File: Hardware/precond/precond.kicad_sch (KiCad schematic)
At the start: 21 parts, among them J1 Conn_Coaxial, J2 Conn_Coaxial, U1 OPA2340, U2 MAX660

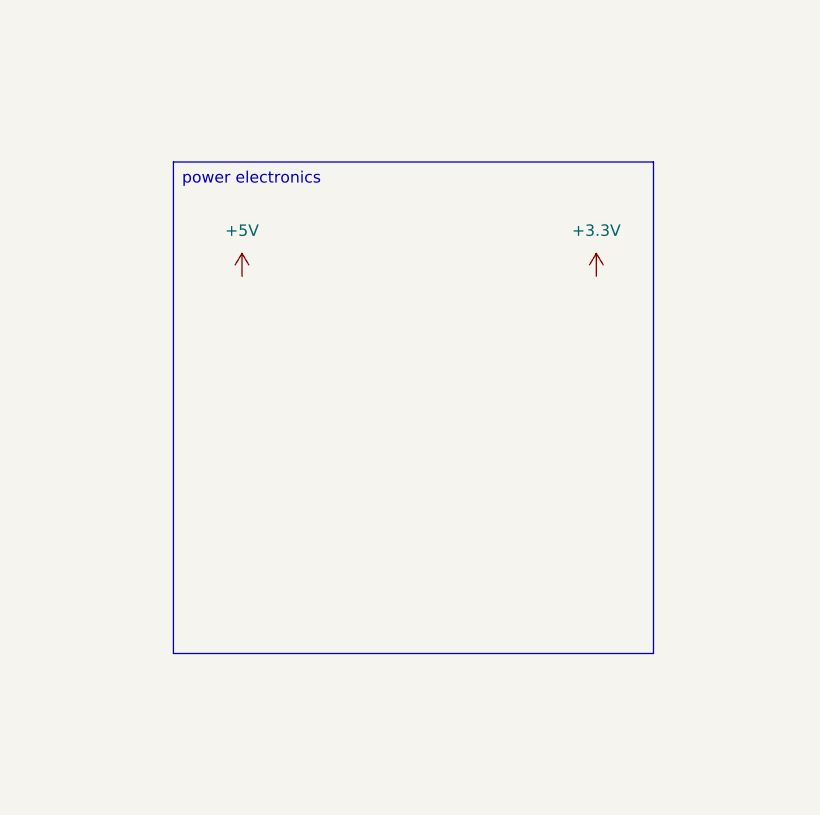
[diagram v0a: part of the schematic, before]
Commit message: buck
buck
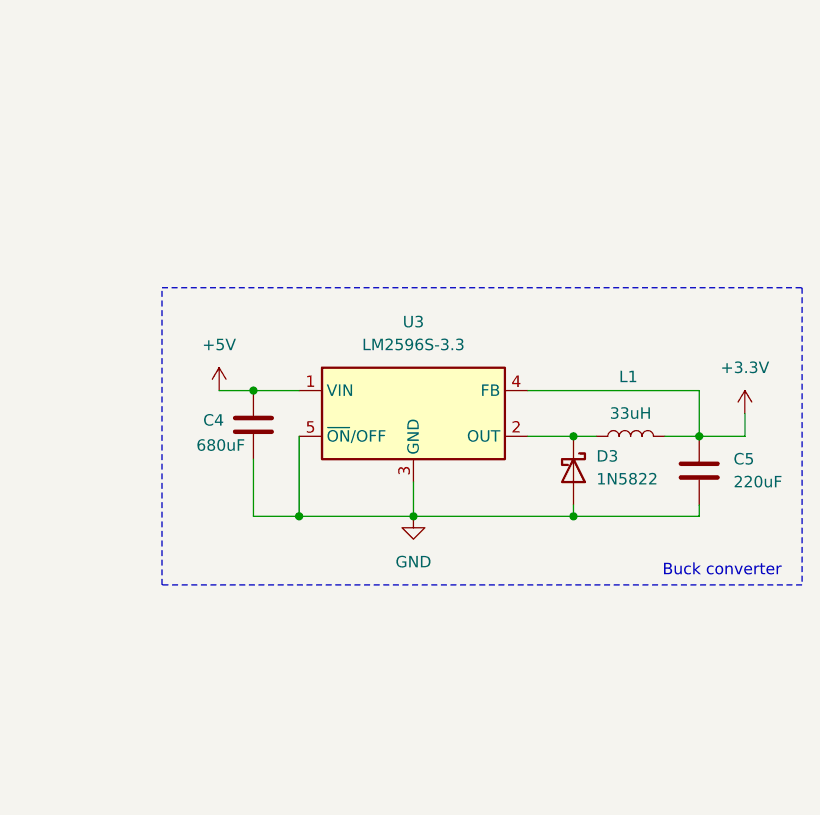
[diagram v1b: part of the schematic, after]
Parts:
- added C4: 680uF, symbol Device:C
- added C5: 220uF, symbol Device:C
- added D3: 1N5822, Diode_THT:D_DO-201AD_P15.24mm_Horizontal, symbol Diode:1N5822
- added L1: 33uH, symbol Device:L
- added U3: LM2596S-3.3, Package_TO_SOT_SMD:TO-263-5_TabPin3, symbol Regulator_Switching:LM2596S-3.3
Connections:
- net +3.3V: now also C5.1, L1.2, U3.4 (FB)
- net +5V: now also C4.1, U3.1 (VIN)
- net GND: now also C4.2, C5.2, D3.2 (A), U3.3 (GND), U3.5 (~{ON}/OFF)
- new net: D3.1 (K), L1.1, U3.2 (OUT)
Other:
- note added: "Buck converter"
